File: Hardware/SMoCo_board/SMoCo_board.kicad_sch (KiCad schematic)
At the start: 47 parts, among them J1 Conn_01x02, J2 Conn_01x02, J4 Conn_01x02, J5 Conn_01x06, J6 Conn_01x02, J7 Conn_01x04, J8 Conn_01x02, Q1 Q_PMOS, U1 STM32F072C8T6, U2 VNH7040AYTR, U3 SN65HVD232, U4 AP63203WU

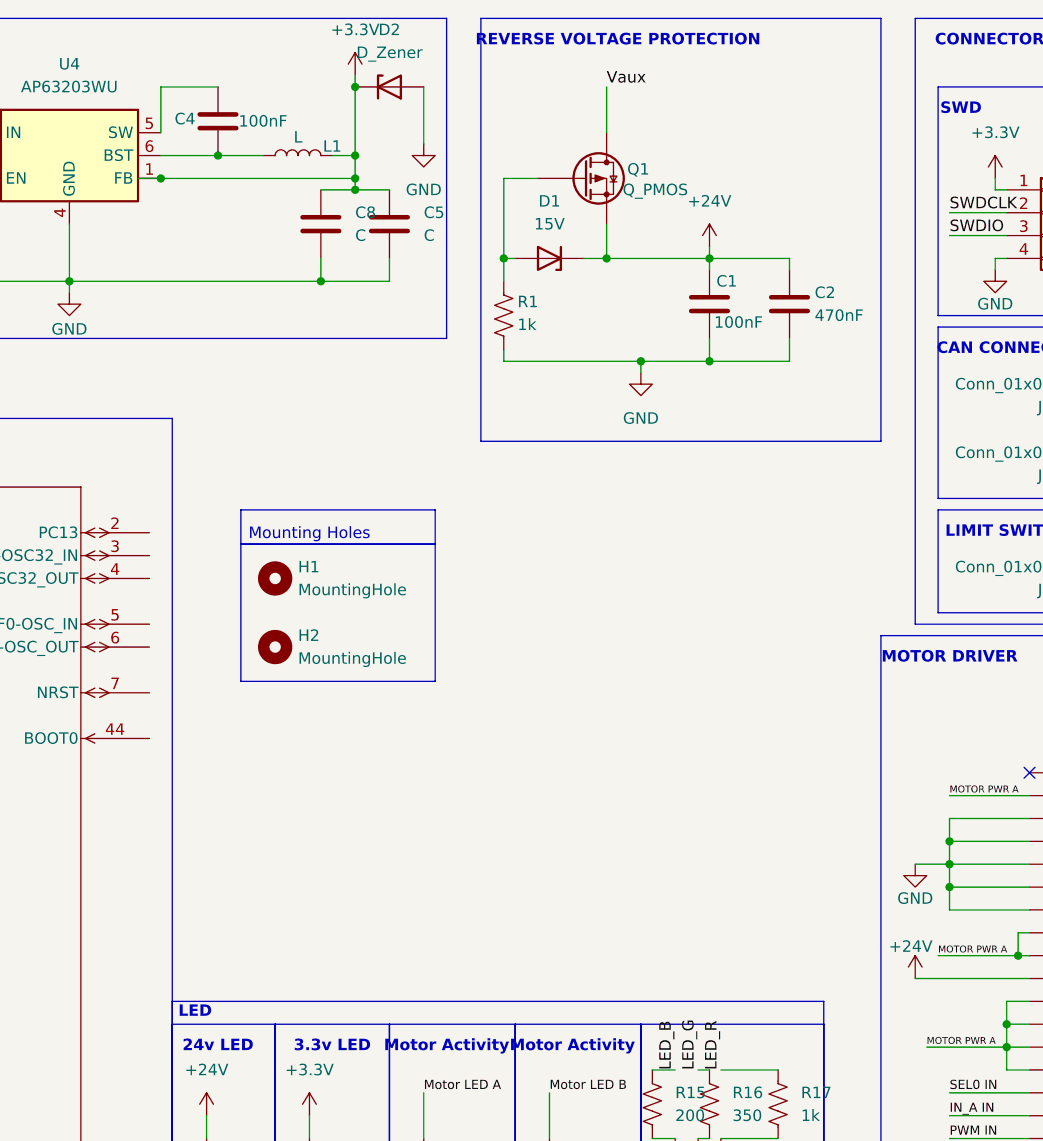
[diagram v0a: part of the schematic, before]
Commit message: SmoCo
update
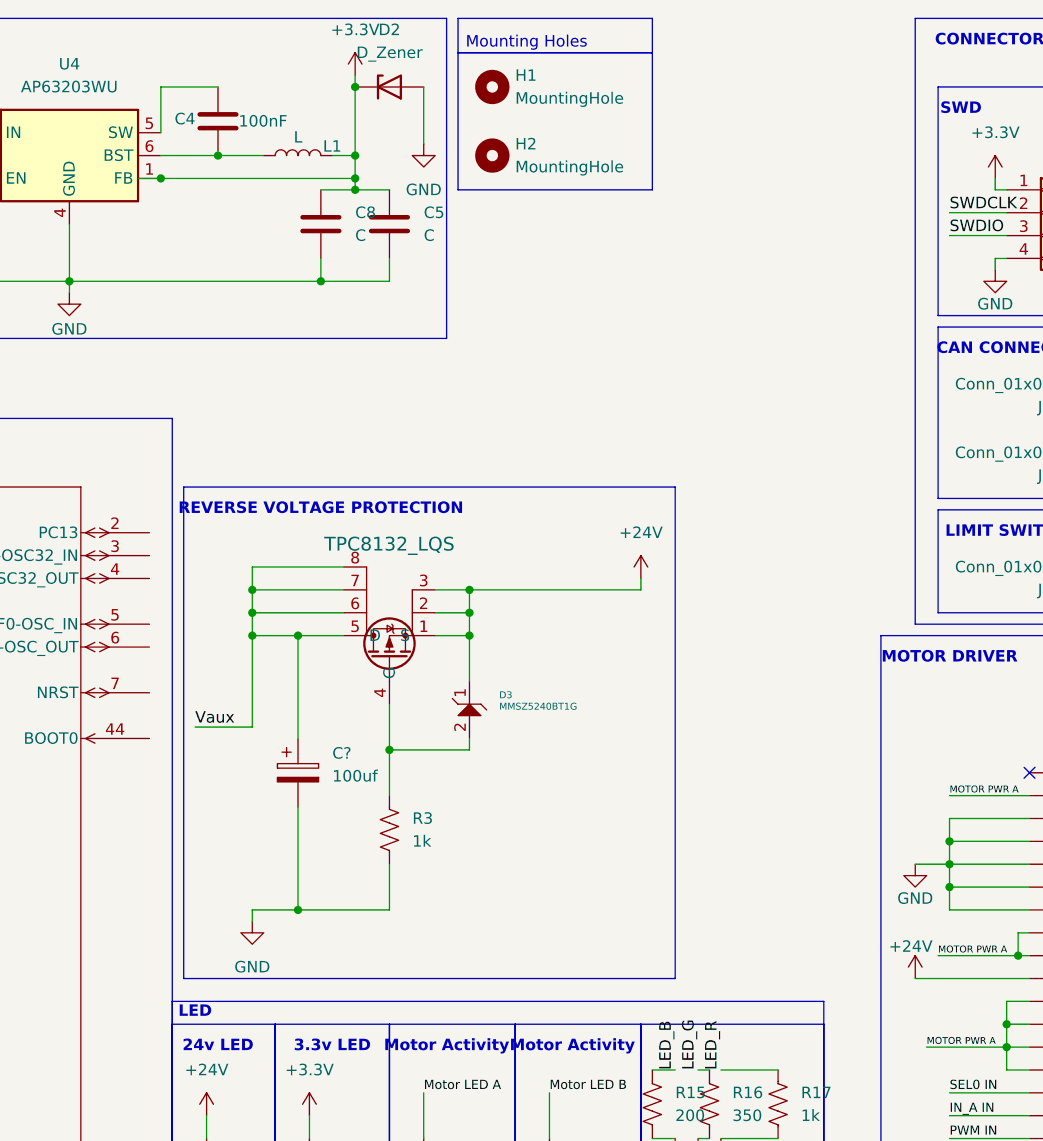
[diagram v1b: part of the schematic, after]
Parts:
- removed C1: 100nF, symbol Device:C
- removed C2: 470nF, symbol Device:C
- removed D1: 15V, symbol Device:D_Zener
- removed Q1: Q_PMOS, symbol Device:Q_PMOS
- removed R1: 1k, symbol Device:R_US
- added C?: 100uf, Capacitor_SMD:C_0603_1608Metric_Pad1.08x0.95mm_HandSolder, symbol Device:C_Polarized
- added D3: MMSZ5240BT1G, MRDT_Devices:SOD-123_ONS-L, symbol MRDT_Devices:MMSZ5240BT1G
- added MOSFET1: TPC8132_LQS, MRDT_Devices:SOP-8_TOS-L, symbol MRDT_Devices:TPC8132_LQS
- added R3: 1k, Resistor_SMD:R_0603_1608Metric_Pad0.98x0.95mm_HandSolder, symbol Device:R_US
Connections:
- net +24V: now also D3.1, MOSFET1.1 (S), MOSFET1.2, MOSFET1.3
- net GND: now also C?.2, R3.2
- net Vaux: now also C?.1, MOSFET1.5 (D), MOSFET1.6, MOSFET1.7, MOSFET1.8
- new net: D3.2, MOSFET1.4 (G), R3.1
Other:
- moved on the sheet: H1, H2
